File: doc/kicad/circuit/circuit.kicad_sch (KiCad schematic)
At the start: 13 parts, among them J1.1 Digital, J1.2 Analog, J2 Handbrake, J3 Encoder, J4 Joystick, J5 Pedals, J6 ATmega328P I²C, J7.1.1 LCD Socket, J7.1.2 PCF8574 LCD Socekt, J7.2 PCF8574 I²C, U1 LCD-016N002L

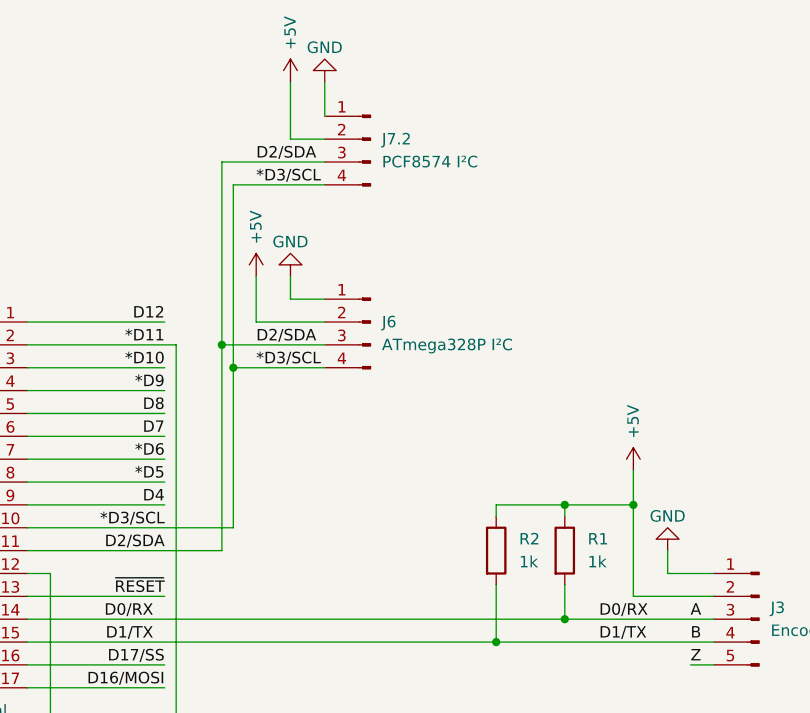
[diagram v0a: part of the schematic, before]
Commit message: start with setup lcd
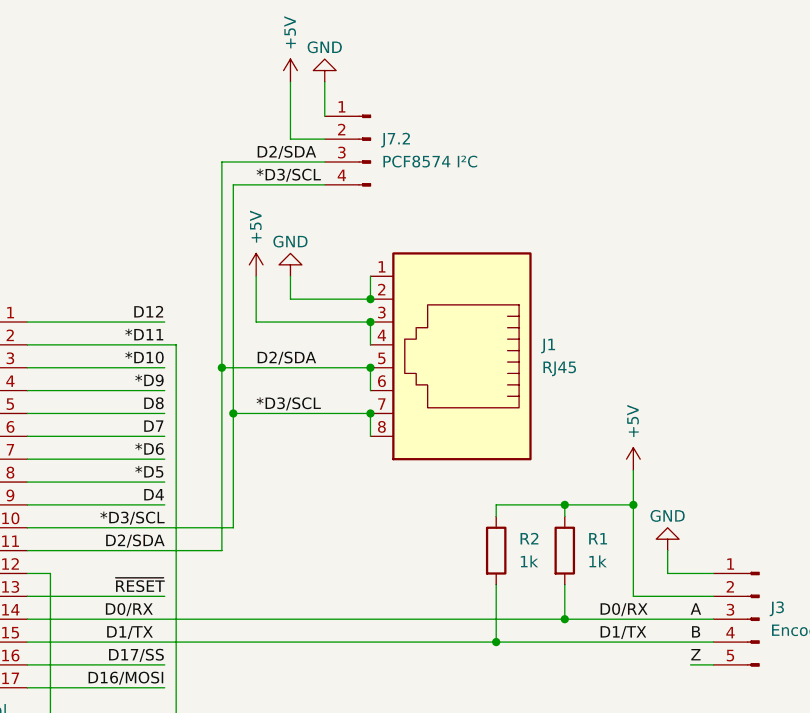
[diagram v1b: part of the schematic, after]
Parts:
- removed J6: ATmega328P I²C, Connector_PinHeader_2.54mm:PinHeader_1x04_P2.54mm_Vertical_SMD_Pin1Left, symbol Connector:Conn_01x04_Pin
- added J1: RJ45, Connector_RJ:RJ45_Molex_0855135013_Vertical, symbol Connector:RJ45
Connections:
- net *D3/SCL: now also J1.7, J1.8
- net +5V: now also J1.3, J1.4
- net D2/SDA: now also J1.5, J1.6
- net GND: now also J1.1, J1.2
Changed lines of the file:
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@@
 	)
 	(junction
-		(at 168.91 121.92)
+		(at 210.82 48.26)
 		(diameter 0)
 		(color 0 0 0 0)
 	)
 	(junction
-		(at 210.82 48.26)
+		(at 210.82 50.8)
 		(diameter 0)
 		(color 0 0 0 0)
 	)
 	(junction
-		(at 210.82 50.8)
+		(at 210.82 38.1)
 		(diameter 0)
 		(color 0 0 0 0)
 	)
 	(junction
-		(at 210.82 38.1)
+		(at 185.42 129.54)
 		(diameter 0)
 		(color 0 0 0 0)
@@
 	)
 	(junction
-		(at 170.18 124.46)
+		(at 168.91 124.46)
 		(diameter 0)
 		(color 0 0 0 0)
@@
 	)
 	(junction
+		(at 170.18 129.54)
+		(diameter 0)
+		(color 0 0 0 0)
+	)
+	(junction
+		(at 185.42 124.46)
+		(diameter 0)
+		(color 0 0 0 0)
+	)
+	(junction
+		(at 185.42 116.84)
+		(diameter 0)
+		(color 0 0 0 0)
+	)
+	(junction
 		(at 210.82 25.4)
 		(diameter 0)
@@
 	)
 	(junction
+		(at 185.42 119.38)
+		(diameter 0)
+		(color 0 0 0 0)
+	)
+	(junction
 		(at 210.82 60.96)
 		(diameter 0)
@@
 	(wire
 		(pts
+			(xy 185.42 114.3) (xy 185.42 116.84)
+		)
+		(stroke
+			(width 0)
+			(type default)
+		)
+	)
+	(wire
+		(pts
 			(xy 260.35 60.96) (xy 237.49 60.96)
 		)
@@
 	(wire
 		(pts
-			(xy 180.34 124.46) (xy 170.18 124.46)
+			(xy 170.18 129.54) (xy 185.42 129.54)
 		)
 		(stroke
@@
 	(wire
 		(pts
+			(xy 185.42 119.38) (xy 185.42 121.92)
+		)
+		(stroke
+			(width 0)
+			(type default)
+		)
+	)
+	(wire
+		(pts
 			(xy 210.82 33.02) (xy 231.14 33.02)
 		)
@@
 	(wire
 		(pts
+			(xy 185.42 129.54) (xy 185.42 132.08)
+		)
+		(stroke
+			(width 0)
+			(type default)
+		)
+	)
+	(wire
+		(pts
 			(xy 62.23 139.7) (xy 127 139.7)
 		)
@@
 	(wire
 		(pts
-			(xy 168.91 121.92) (xy 180.34 121.92)
+			(xy 168.91 124.46) (xy 185.42 124.46)
 		)
 		(stroke
@@
 	(wire
 		(pts
+			(xy 170.18 104.14) (xy 170.18 129.54)
+		)
+		(stroke
+			(width 0)
+			(type default)
+		)
+	)
+	(wire
+		(pts
 			(xy 214.63 149.86) (xy 223.52 149.86)
 		)
@@
 	(wire
 		(pts
+			(xy 185.42 124.46) (xy 185.42 127)
+		)
+		(stroke
+			(width 0)
+			(type default)
+		)
+	)
+	(wire
+		(pts
 			(xy 180.34 99.06) (xy 176.53 99.06)
 		)
@@
 	(wire
 		(pts
+			(xy 168.91 124.46) (xy 168.91 144.78)
+		)
+		(stroke
+			(width 0)
+			(type default)
+		)
+	)
+	(wire
+		(pts
 			(xy 214.63 139.7) (xy 214.63 135.89)
 		)
@@
 	(wire
 		(pts
-			(xy 168.91 101.6) (xy 168.91 121.92)
-		)
-		(stroke
-			(width 0)
-			(type default)
-		)
-	)
-	(wire
-		(pts
 			(xy 232.41 35.56) (xy 210.82 35.56)
 		)
@@
 	(wire
 		(pts
+			(xy 170.18 129.54) (xy 170.18 142.24)
+		)
+		(stroke
+			(width 0)
+			(type default)
+		)
+	)
+	(wire
+		(pts
 			(xy 200.66 33.02) (xy 210.82 33.02)
 		)
@@
 	(wire
 		(pts
-			(xy 180.34 119.38) (xy 172.72 119.38)
+			(xy 172.72 119.38) (xy 185.42 119.38)
 		)
 		(stroke
@@
 	(wire
 		(pts
-			(xy 176.53 116.84) (xy 180.34 116.84)
+			(xy 176.53 116.84) (xy 185.42 116.84)
 		)
 		(stroke
@@
 	(wire
 		(pts
-			(xy 168.91 121.92) (xy 168.91 144.78)
+			(xy 168.91 101.6) (xy 168.91 124.46)
 		)
 		(stroke
@@
 	(wire
 		(pts
-			(xy 170.18 124.46) (xy 170.18 142.24)
-		)
-		(stroke
-			(width 0)
-			(type default)
-		)
-	)
-	(wire
-		(pts
 			(xy 124.46 152.4) (xy 124.46 165.1)
 		)
@@
 	(wire
 		(pts
-			(xy 170.18 104.14) (xy 170.18 124.46)
-		)
-		(stroke
-			(width 0)
-			(type default)
-		)
-	)
-	(wire
-		(pts
 			(xy 176.53 99.06) (xy 176.53 92.71)
 		)
@@
 	)
 	(label "*D3{slash}SCL"
-		(at 172.72 124.46 0)
+		(at 172.72 129.54 0)
 		(fields_autoplaced yes)
 		(effects
@@
 	)
 	(label "D2{slash}SDA"
-		(at 172.72 121.92 0)
+		(at 172.72 124.46 0)
 		(fields_autoplaced yes)
 		(effects
@@
 	)
 	(symbol
-		(lib_id "Connector:Conn_01x04_Pin")
-		(at 185.42 119.38 0)
-		(mirror y)
-		(unit 1)
-		(exclude_from_sim no)
-		(in_bom yes)
-		(on_board yes)
-		(dnp no)
-		(fields_autoplaced yes)
-		(property "Reference" "J6"
-			(at 186.69 119.3799 0)
-			(effects
-				(font
-					(size 1.27 1.27)
-				)
-				(justify right)
-			)
-		)
-		(property "Value" "ATmega328P I²C"
-			(at 186.69 121.9199 0)
-			(effects
-				(font
-					(size 1.27 1.27)
-				)
-				(justify right)
-			)
-		)
-		(property "Footprint" "Connector_PinHeader_2.54mm:PinHeader_1x04_P2.54mm_Vertical_SMD_Pin1Left"
-			(at 185.42 119.38 0)
-			(effects
-				(font
-					(size 1.27 1.27)
-				)
-				(hide yes)
-			)
-		)
-		(property "Datasheet" "~"
-			(at 185.42 119.38 0)
-			(effects
-				(font
-					(size 1.27 1.27)
-				)
-				(hide yes)
-			)
-		)
-		(property "Description" "Generic connector, single row, 01x04, script generated"
-			(at 185.42 119.38 0)
-			(effects
-				(font
-					(size 1.27 1.27)
-				)
-				(hide yes)
-			)
-		)
-		(pin "2"
-		)
-		(pin "3"
-		)
-		(pin "1"
-		)
-		(pin "4"
-		)
-		(instances
-			(project ""
-				(path "/e63e39d7-6ac0-4ffd-8aa3-1841a4541b55"
-					(reference "J6")
-					(unit 1)
-				)
-			)
-		)
-	)
-	(symbol
 		(lib_id "Connector:Conn_01x03_Pin")
 		(at 77.47 132.08 0)
@@
 					(unit 1)
 				)
+			)
+		)
+	)
+	(symbol
+		(lib_id "Connector:RJ45")
+		(at 195.58 121.92 180)
+		(unit 1)
+		(exclude_from_sim no)
+		(in_bom yes)
+		(on_board yes)
+		(dnp no)
+		(fields_autoplaced yes)
+		(property "Reference" "J1"
+			(at 204.47 121.9199 0)
+			(effects
+				(font
+					(size 1.27 1.27)
+				)
+				(justify right)
+			)
+		)
+		(property "Value" "RJ45"
+			(at 204.47 124.4599 0)
+			(effects
+				(font
+					(size 1.27 1.27)
+				)
+				(justify right)
+			)
+		)
+		(property "Footprint" "Connector_RJ:RJ45_Molex_0855135013_Vertical"
+			(at 195.58 122.555 90)
+			(effects
+				(font
+					(size 1.27 1.27)
+				)
+				(hide yes)
+			)
+		)
+		(property "Datasheet" "~"
+			(at 195.58 122.555 90)
+			(effects
+				(font
+					(size 1.27 1.27)
+				)
+				(hide yes)
+			)
+		)
+		(property "Description" "RJ connector, 8P8C (8 positions 8 connected)"
+			(at 195.58 121.92 0)
+			(effects
+				(font
+					(size 1.27 1.27)
+				)
+				(hide yes)
+			)
+		)
+		(pin "4"
+		)
+		(pin "6"
+		)
+		(pin "2"
+		)
+		(pin "3"
+		)
+		(pin "8"
+		)
+		(pin "7"
+		)
+		(pin "5"
+		)
+		(pin "1"
+		)
+		(instances
+			(project ""
+				(path "/e63e39d7-6ac0-4ffd-8aa3-1841a4541b55"
+					(reference "J1")
+					(unit 1)
+				)
